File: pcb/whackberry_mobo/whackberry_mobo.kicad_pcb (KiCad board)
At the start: 2 copper layers, 14 parts, among them J1 GroveFemaleHeader_114020164, J2 USBa_Port_87583-0010BHLF, SW1 SW_Omron_B3FS, SW2 SW_Omron_B3FS, U2 TSOP348xx, U5 2232_display

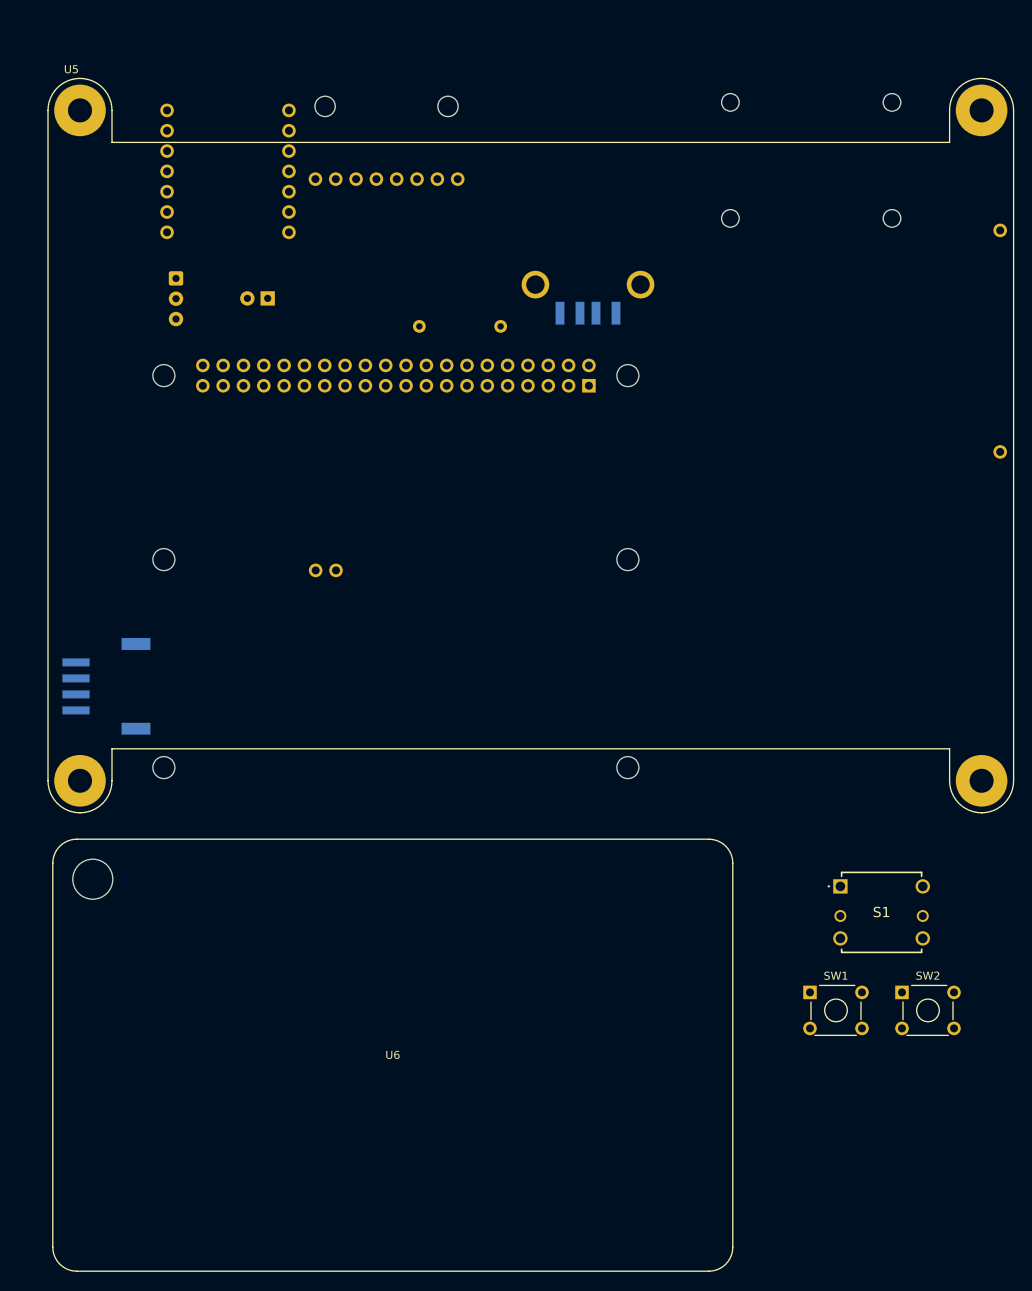
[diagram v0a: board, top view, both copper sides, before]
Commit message: Ready for tracing PCB
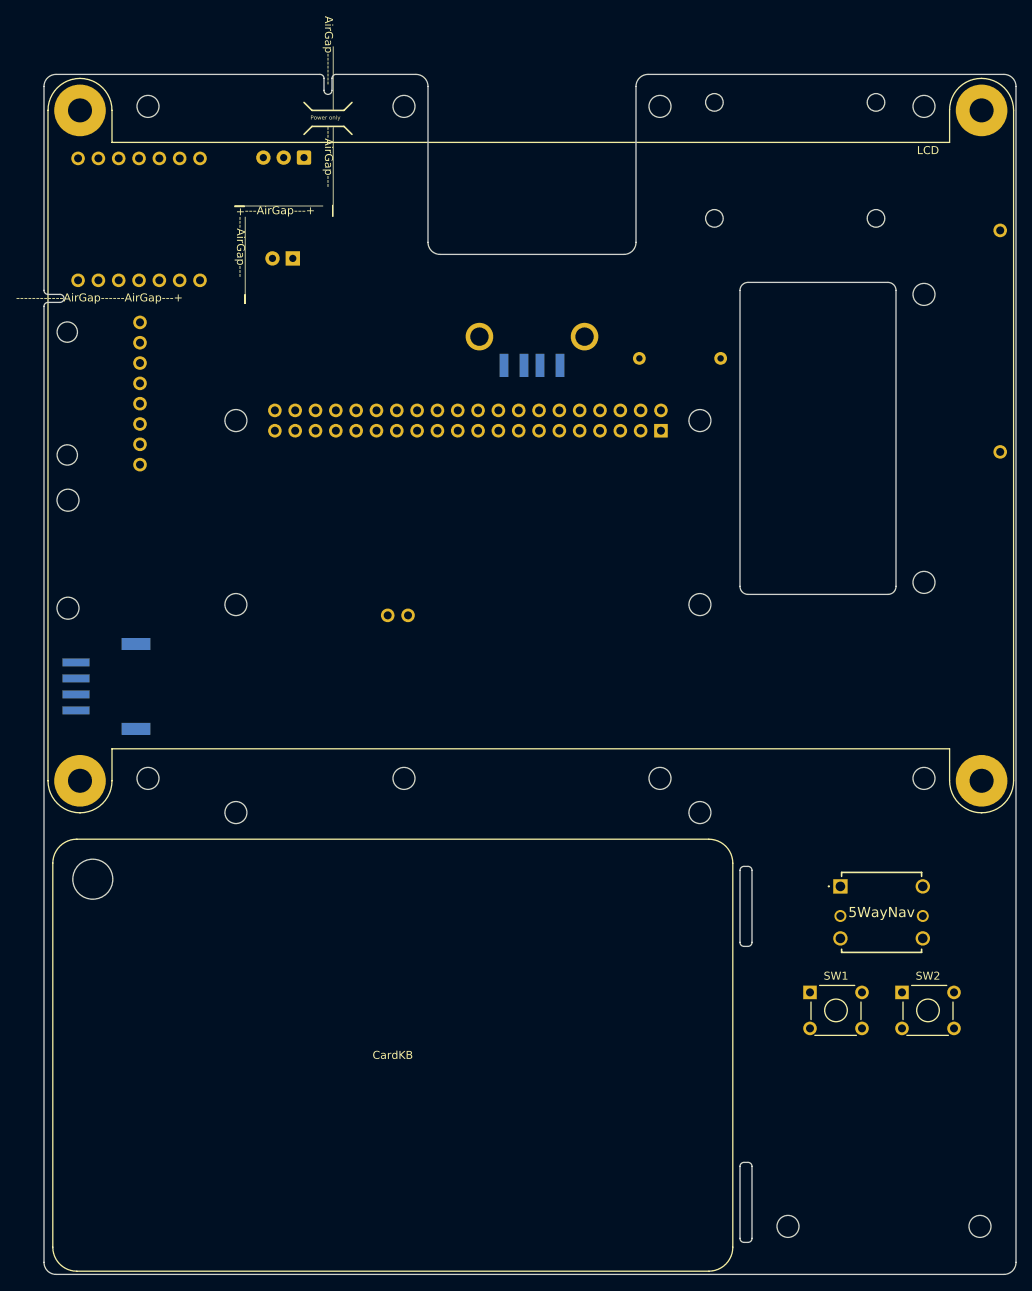
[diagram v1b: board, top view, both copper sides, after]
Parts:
- moved USB-C 37.6 mm to (55.1, 72.9), turned to -90 degrees
- moved QTpy 30.3 mm to (37.2, 37.1), turned to -90 degrees
- moved R1 27.8 mm to (122.6, 54.5)
- moved IR-Re 22.0 mm to (70.5, 29.4), turned to 180 degrees
- moved RPi-Zero 10.6 mm to (65.1, 63.5)
- moved USB-A 9.55 mm to (99.0, 48.5)
- moved IR-LED 5.90 mm to (69.1, 42.0)
- moved Camera 2.00 mm to (109.4, 34.1)
- renumbered S1 to 5WayNav, U4 to Camera, U6 to CardKB, J1 to GROVE, D1 to IR-LED, U2 to IR-Re, U5 to LCD, U3 to QTpy, U1 to RPi-Zero, J2 to USB-A, U7 to USB-C
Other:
- board outline added: 121.5 x 150 mm
- board text added: "+---AirGap---"
- board text added: "+---AirGap------AirGap-----------"
- board text added: "------------AirGap------AirGap---+"
- board text added: "--------AirGap"
- board text added: "---AirGap---"
- board text added: "---AirGap---+"
- board text added: "AirGap--------"
- board text added: "Power only"
